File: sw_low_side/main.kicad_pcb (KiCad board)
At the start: 2 copper layers, 76.2 x 17.8 mm, 9 parts, among them P1 CONN_XT60, P2 CONN_XT60, P3 CONN_01X02, Q1 IRFB7537PbF, U1 NSI45020AT1G, U2 LM3490IM5-12/NOPB

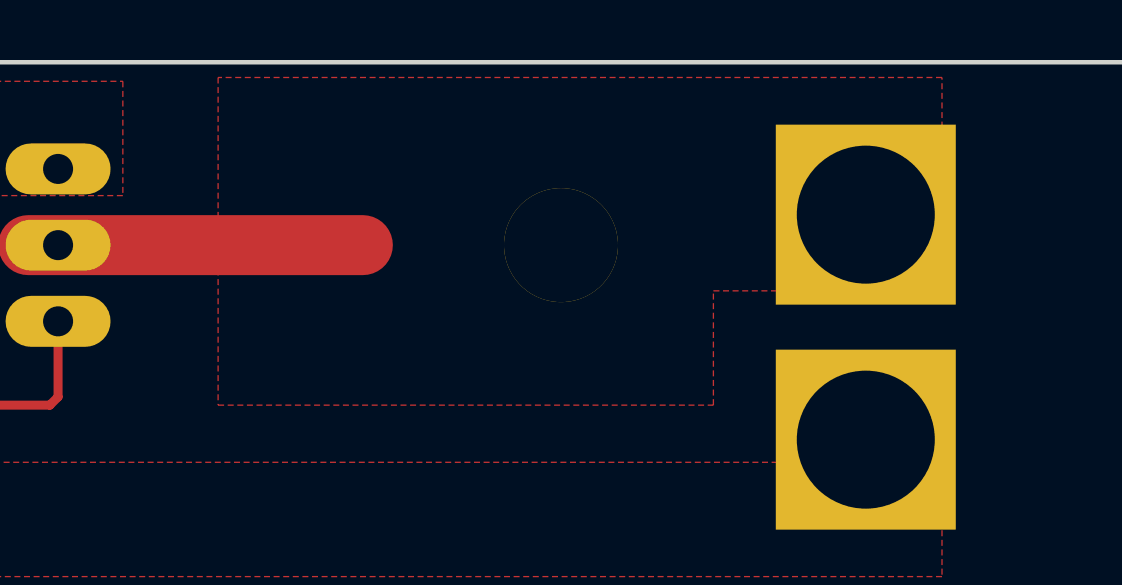
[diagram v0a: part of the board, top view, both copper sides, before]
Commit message: test
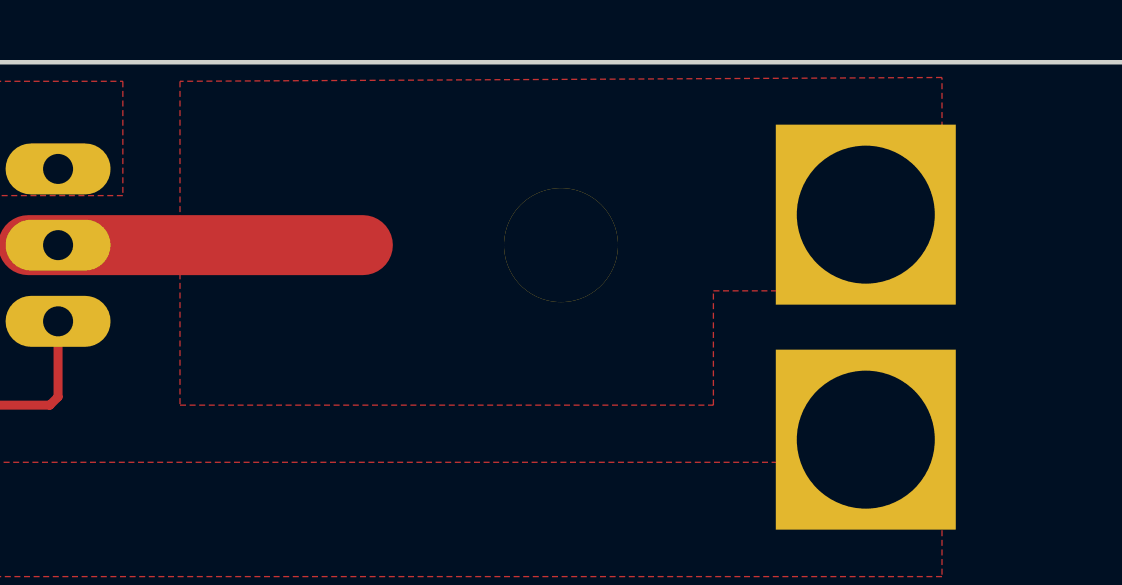
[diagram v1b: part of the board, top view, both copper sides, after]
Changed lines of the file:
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@@
   )
   (setup
-    (last_trace_width 1)
+    (last_trace_width 0.25)
     (user_trace_width 0.3)
     (user_trace_width 0.4)
@@
     (polygon
       (pts
-        (xy 168.91 132.588) (xy 168.91 143.51) (xy 185.42 143.51) (xy 185.42 139.7) (xy 193.04 139.7)
+        (xy 167.64 132.715) (xy 167.64 143.51) (xy 185.42 143.51) (xy 185.42 139.7) (xy 193.04 139.7)
         (xy 193.04 132.588)
       )
